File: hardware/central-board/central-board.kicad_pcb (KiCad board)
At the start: 2 copper layers, 65 x 56 mm, 64 parts, among them J1 MTJ-88ARX1-FSM-LG, J10 Conn_01x02, J11 Conn_01x02, J12 IO I2C Bus, J2 1729128, J3 1729128, J4 RPi_GPIO, J5 PEC11R, J6 IO Power Bus, J7 GPIO Bus, J8 Conn_01x02, Q1 AO3400A, Q2 AO3400A, Q3 AO3400A, Q4 AO3400A, Q5 AO3400A, Q6 AO3400A, U1 MAX3485, U4 TPS5430DDAR, U5 XC6220B331MR, U6 TPS5430DDAR

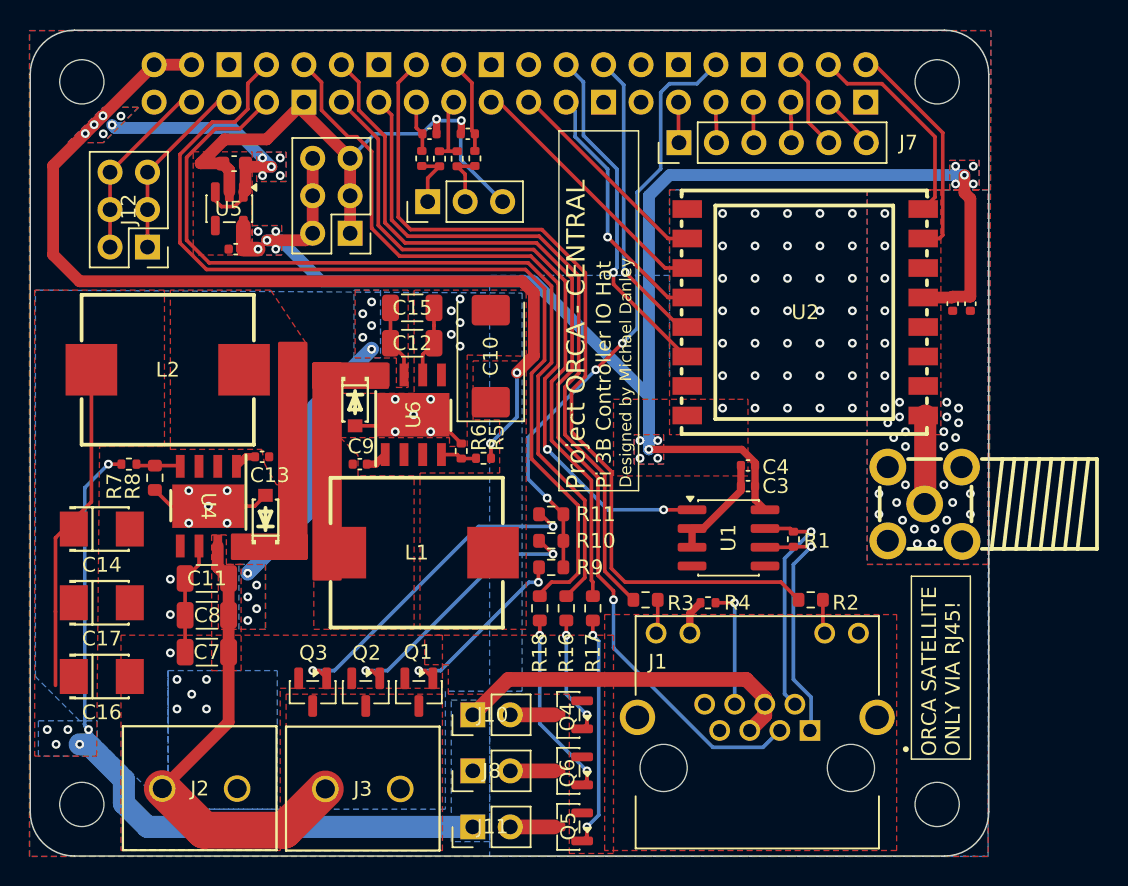
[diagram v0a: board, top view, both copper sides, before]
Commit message: Prepared for production
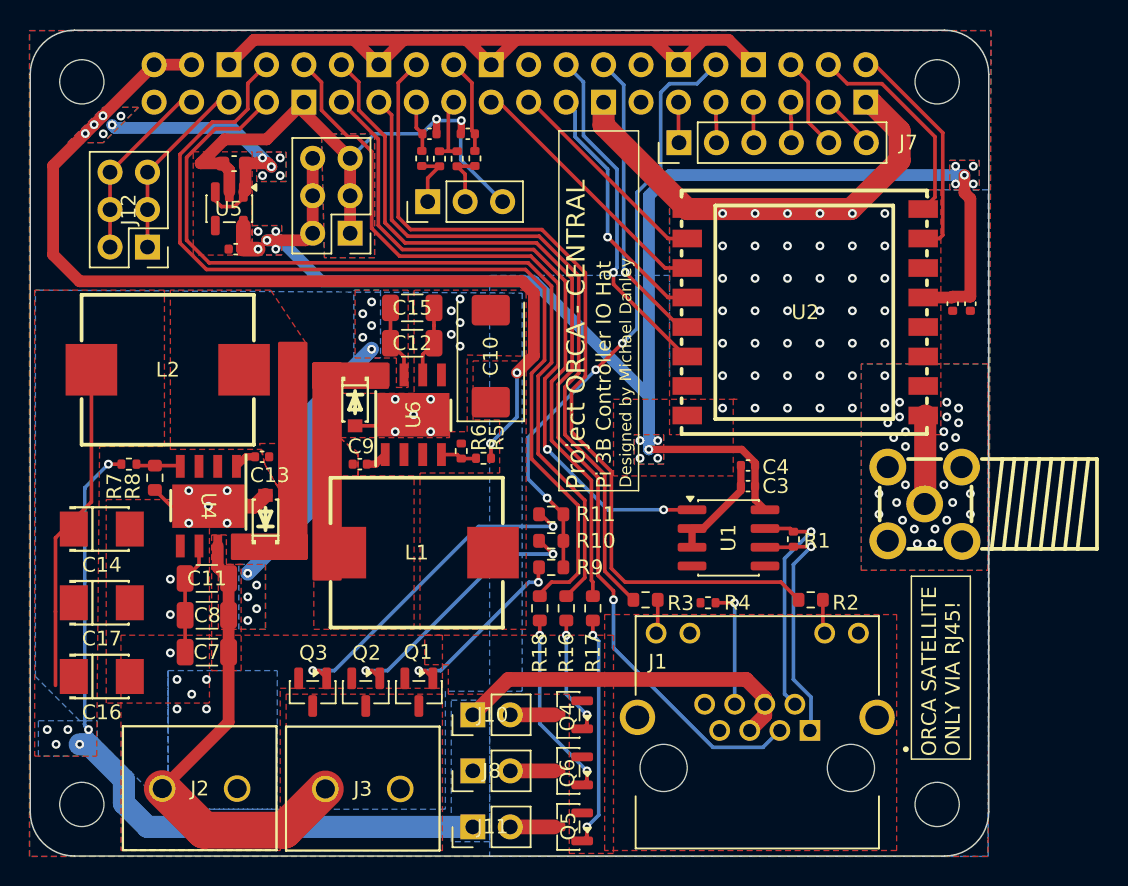
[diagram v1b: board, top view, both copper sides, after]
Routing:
- net GND: track 78.9 -> 155.5 mm
